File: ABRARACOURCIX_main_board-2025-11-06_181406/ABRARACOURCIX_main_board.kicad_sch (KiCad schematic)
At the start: 6 parts, among them U1 STM32F429ZIT6

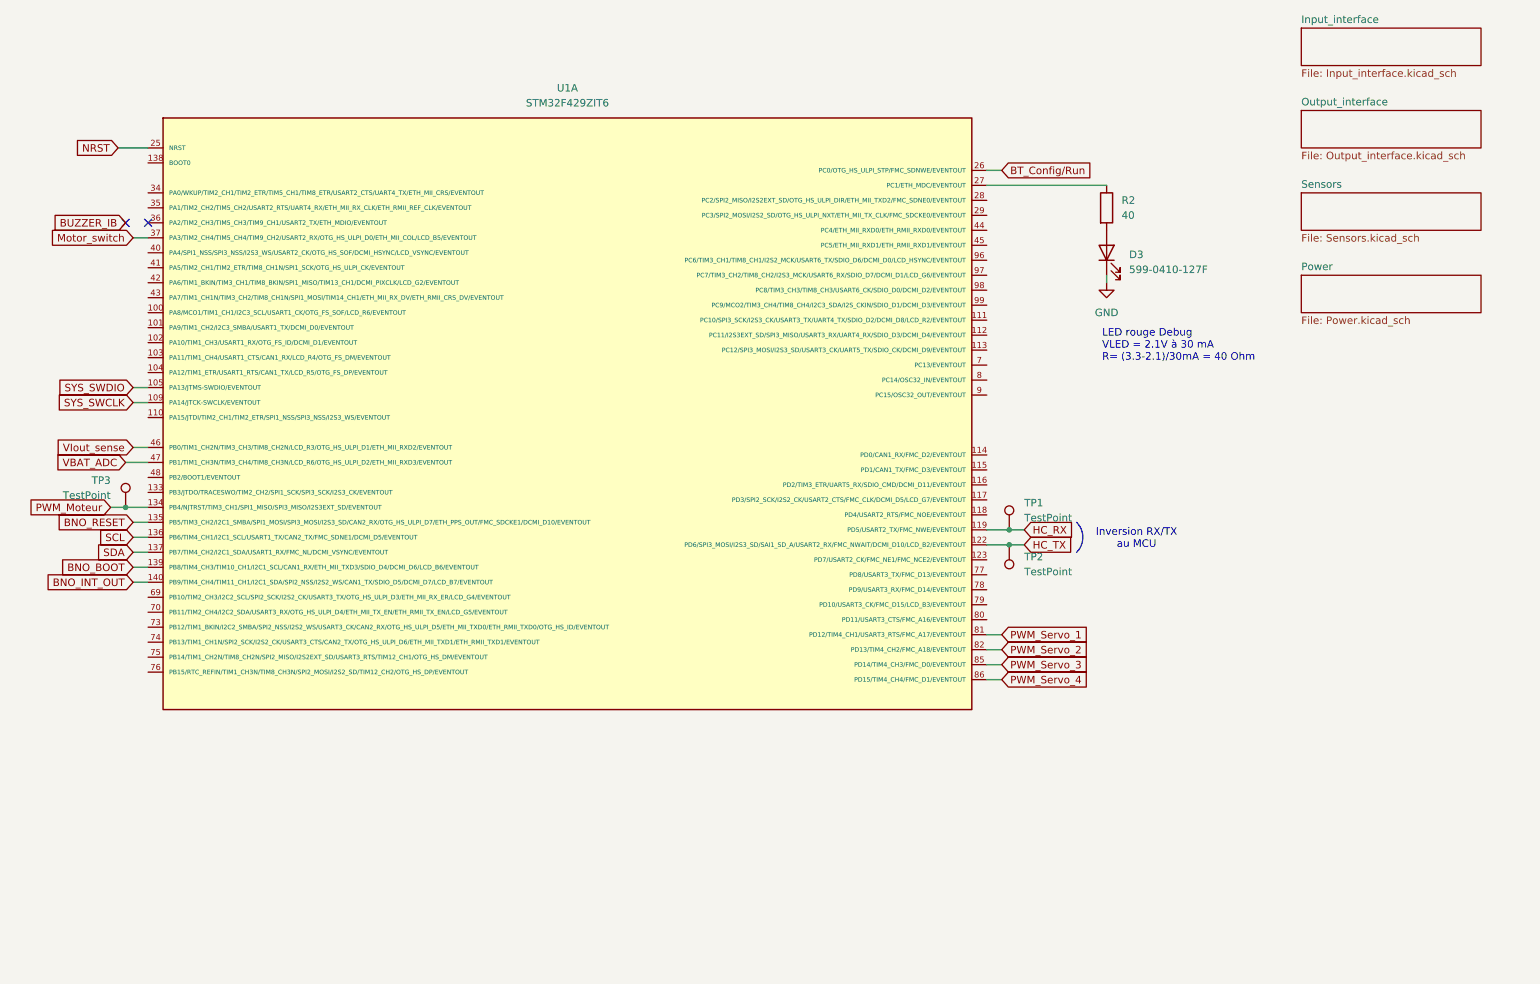
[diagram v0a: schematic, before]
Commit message: Modifs au circuit d'alim
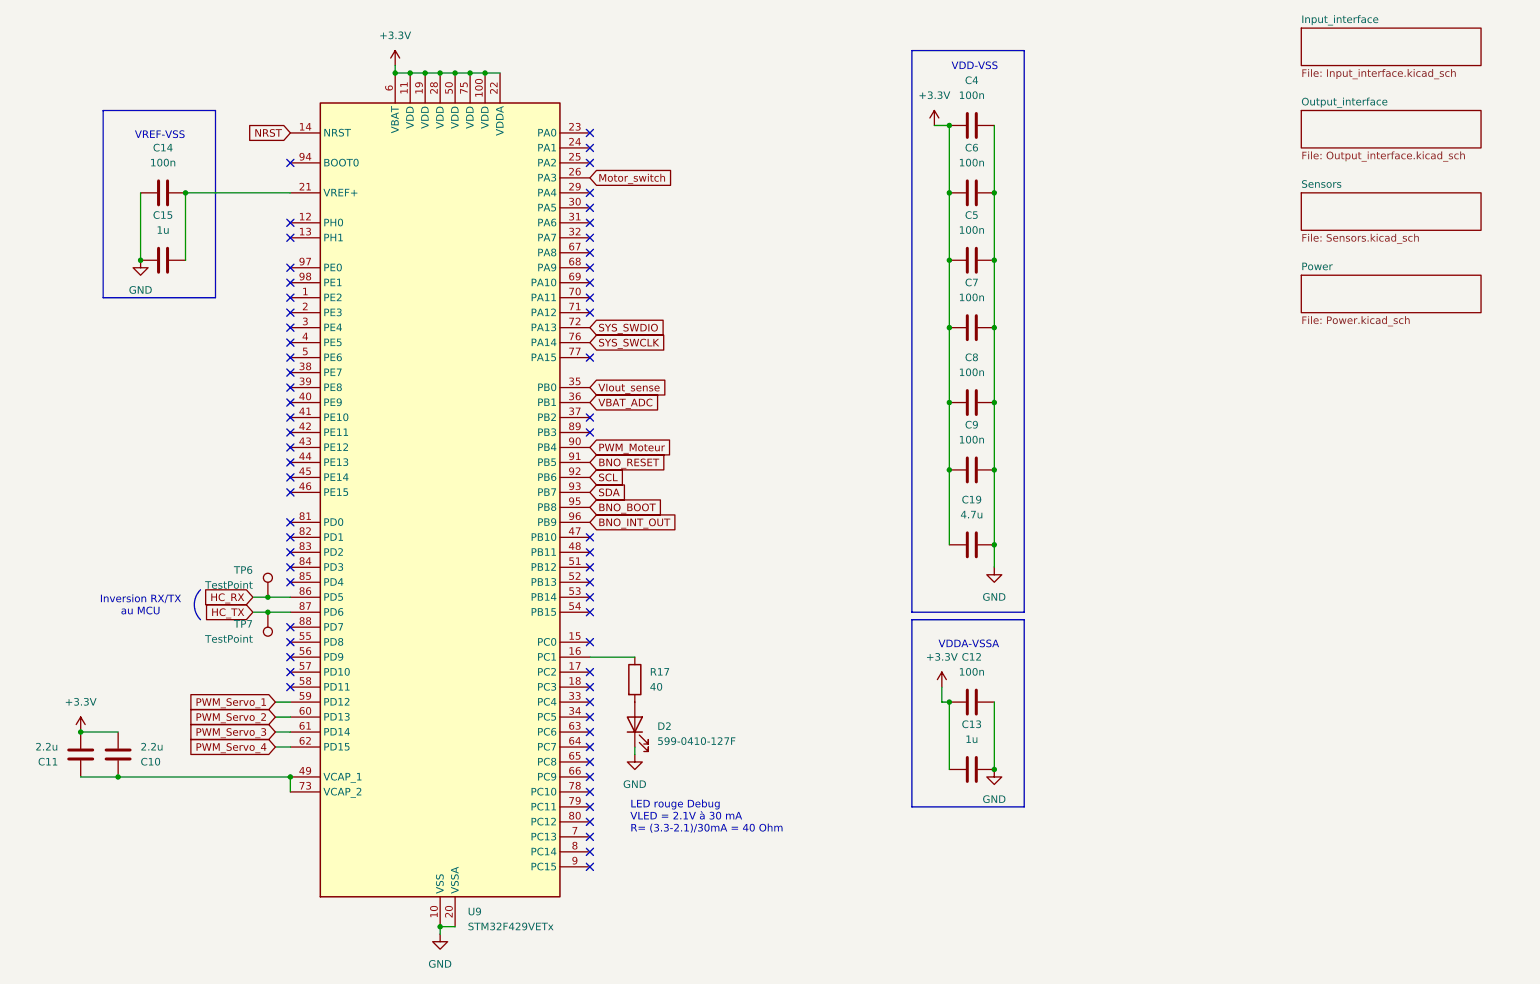
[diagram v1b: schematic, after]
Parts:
- removed D3: 599-0410-127F, Diode_SMD:D_1206_3216Metric_Pad1.42x1.75mm_HandSolder, symbol Device:LED
- removed R2: 40, Resistor_SMD:R_1206_3216Metric_Pad1.30x1.75mm_HandSolder, symbol Device:R
- removed TP1, TP2, TP3: TestPoint, TestPoint:TestPoint_THTPad_2.0x2.0mm_Drill1.0mm, symbol Connector:TestPoint
- removed U1: STM32F429ZIT6, Librairie_footprint:QFP50P2200X2200X160-144N, symbol GAUL_ABRARACOURCIX:STM32F429ZIT6
- added C10, C11: 2.2u, Capacitor_SMD:C_1206_3216Metric_Pad1.33x1.80mm_HandSolder, symbol Device:C
- added C12, C14, C4, C5, C6, C7, C8, C9: 100n, Capacitor_SMD:C_1206_3216Metric_Pad1.33x1.80mm_HandSolder, symbol Device:C
- added C13, C15: 1u, Capacitor_SMD:C_1206_3216Metric_Pad1.33x1.80mm_HandSolder, symbol Device:C
- added C19: 4.7u, Capacitor_SMD:C_1206_3216Metric_Pad1.33x1.80mm_HandSolder, symbol Device:C
- added D2: 599-0410-127F, Diode_SMD:D_1206_3216Metric_Pad1.42x1.75mm_HandSolder, symbol Device:LED
- added R17: 40, Resistor_SMD:R_1206_3216Metric_Pad1.30x1.75mm_HandSolder, symbol Device:R
- added TP6, TP7: TestPoint, TestPoint:TestPoint_THTPad_2.0x2.0mm_Drill1.0mm, symbol Connector:TestPoint
- added U9: STM32F429VETx, Package_QFP:LQFP-100_14x14mm_P0.5mm, symbol MCU_ST_STM32F4:STM32F429VETx
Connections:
- net BNO_BOOT: now also U9.95 (PB8)
- net BNO_INT_OUT: now also U9.96 (PB9)
- net BNO_RESET: now also U9.91 (PB5)
- net GND: now also C12.2, C13.2, C14.1, C15.1, C19.2, C4.2, C5.2, C6.2, C7.2, C8.2, C9.2, D2.1 (K), U9.10 (VSS), U9.20 (VSSA), U9.27 (VSS), U9.74 (VSS), U9.99 (VSS)
- net HC_RX: now also TP6.1, U9.86 (PD5)
- net HC_TX: now also TP7.1, U9.87 (PD6)
- net Motor_switch: now also U9.26 (PA3)
- net NRST: now also U9.14 (NRST)
- net PWM_Moteur: now also U9.90 (PB4)
- net PWM_Servo_1: now also U9.59 (PD12)
- net PWM_Servo_2: now also U9.60 (PD13)
- net PWM_Servo_3: now also U9.61 (PD14)
- net PWM_Servo_4: now also U9.62 (PD15)
- net SCL: now also U9.92 (PB6)
- net SDA: now also U9.93 (PB7)
- net SYS_SWCLK: now also U9.76 (PA14)
- net SYS_SWDIO: now also U9.72 (PA13)
- net VBAT_ADC: now also U9.36 (PB1)
- net VIout_sense: now also U9.35 (PB0)
- new net: C10.1, C11.1, U9.49 (VCAP_1), U9.73 (VCAP_2)
- new net: D2.2 (A), R17.2
- new net: R17.1, U9.16 (PC1)
- new net: C14.2, C15.2, U9.21 (VREF+)
- new net +3.3V: C10.2, C11.2, C12.1, C13.1, C19.1, C4.1, C5.1, C6.1, C7.1, C8.1, C9.1, U9.100 (VDD), U9.11 (VDD), U9.19 (VDD), U9.22 (VDDA), U9.28 (VDD), U9.50 (VDD), U9.6 (VBAT), U9.75 (VDD)
- no-connect marks 2 -> 65
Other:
- note added: "VDD-VSS"
- note added: "VDDA-VSSA"
- note added: "VREF-VSS"
